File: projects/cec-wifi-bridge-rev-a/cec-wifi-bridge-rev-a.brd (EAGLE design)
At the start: 75.9 x 36.1 mm, 56 parts, among them J1 DX4R005HJ5R2000, J3 DEBUG, J4 10029449-001RLF, J5 PROGRAM, T1 MMBT3904, T2 MMBT3904, U1 MCP73831/2/OT, U2 TPS61200DRC, U3 ESP8266EX, U4 SPI-FLASH-SOIC8, X1 26MHz

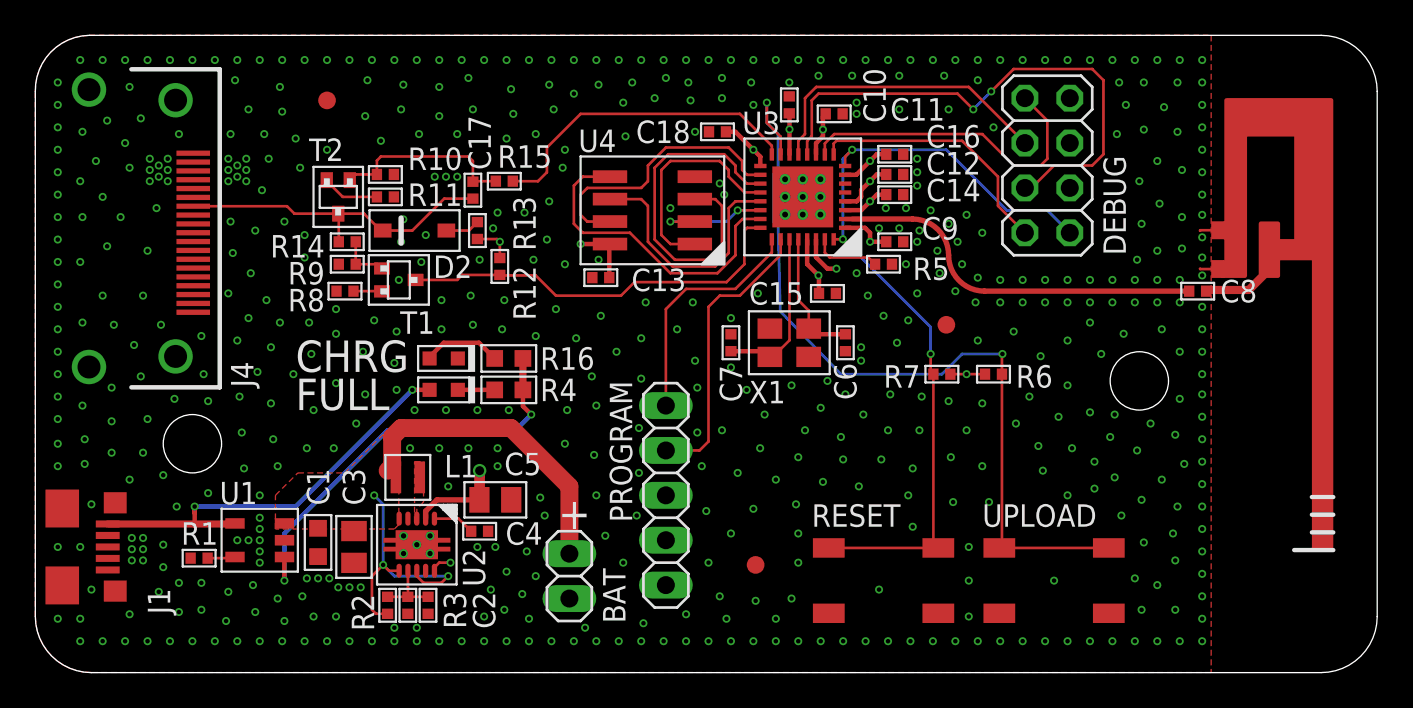
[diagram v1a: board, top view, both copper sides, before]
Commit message: More sane stitching.
The stitching before was haphazard, ugly, overkill, and generally
wasteful.  I did a more sane and uniform stitching of ground.

Looks better, and I'm guessing things will function just the same.
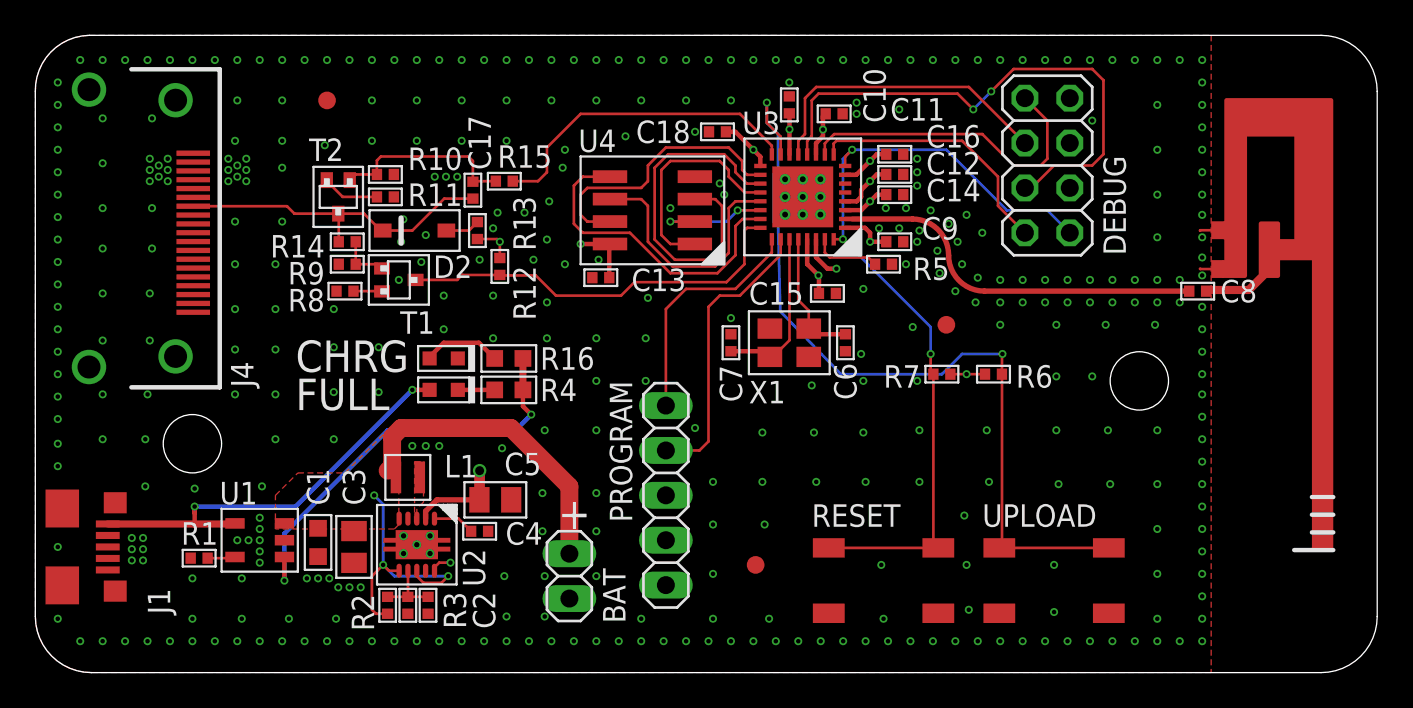
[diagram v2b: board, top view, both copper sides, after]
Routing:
- net AGND: vias 567 -> 387
